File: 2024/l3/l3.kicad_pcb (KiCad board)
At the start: 2 copper layers, 137.5 x 129.1 mm, 23 parts, among them J1 Conn_01x04, SW1 SW_SPDT, SW2 SW_SPDT, SW3 SW_SPDT, SW4 SW_SPDT, U4 DEV-15583

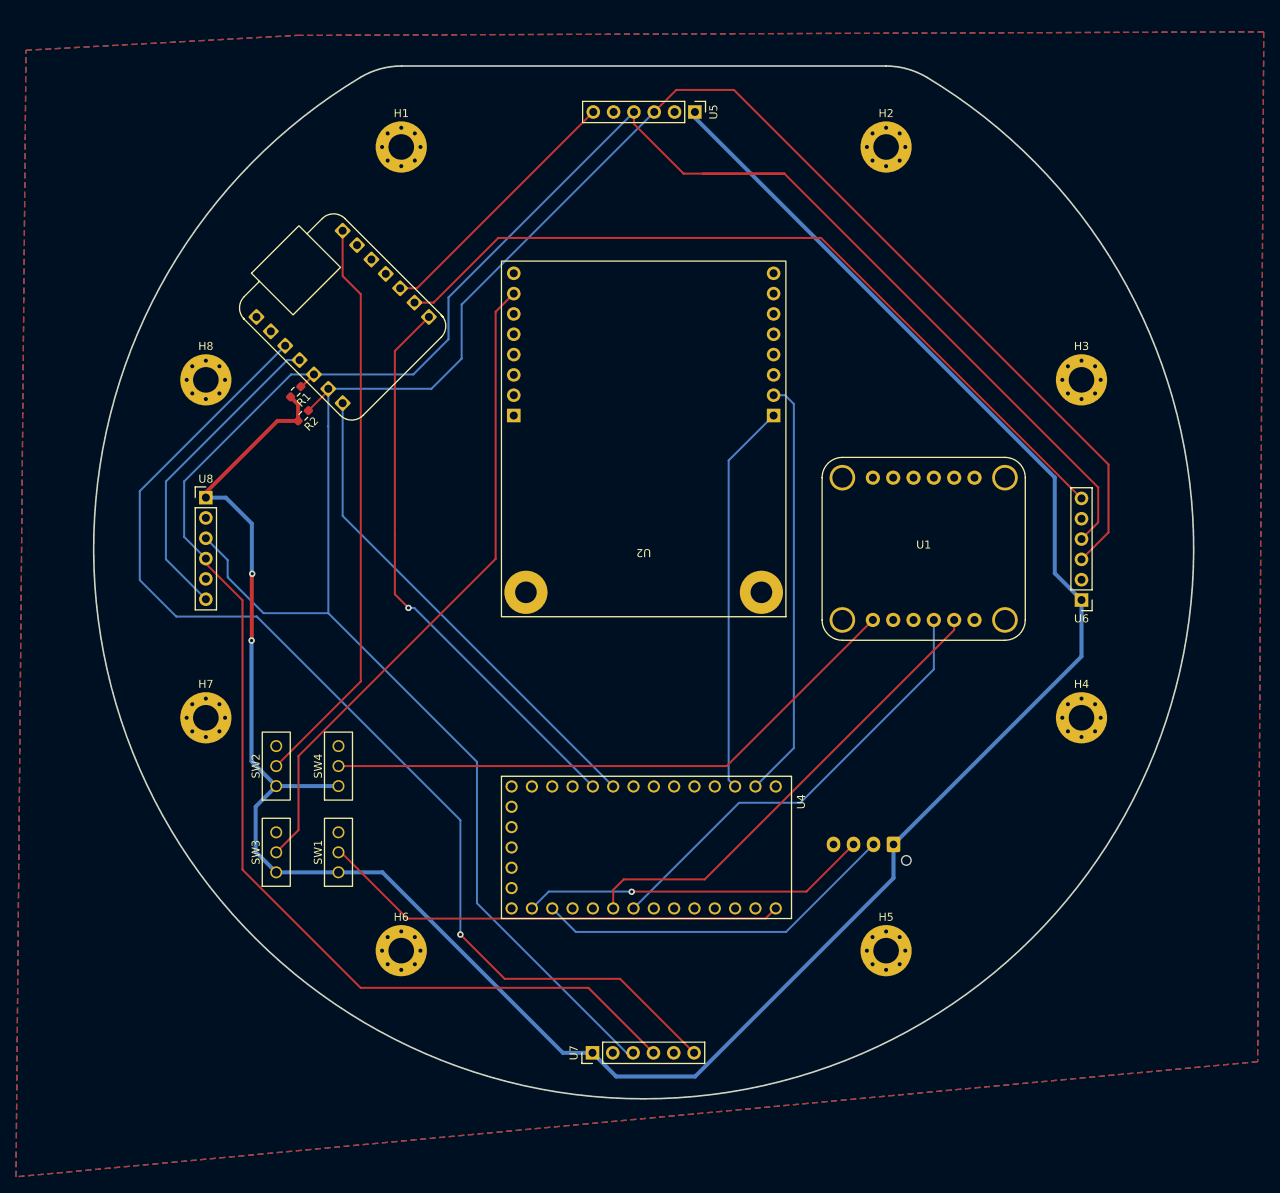
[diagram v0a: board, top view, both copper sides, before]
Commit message: nose
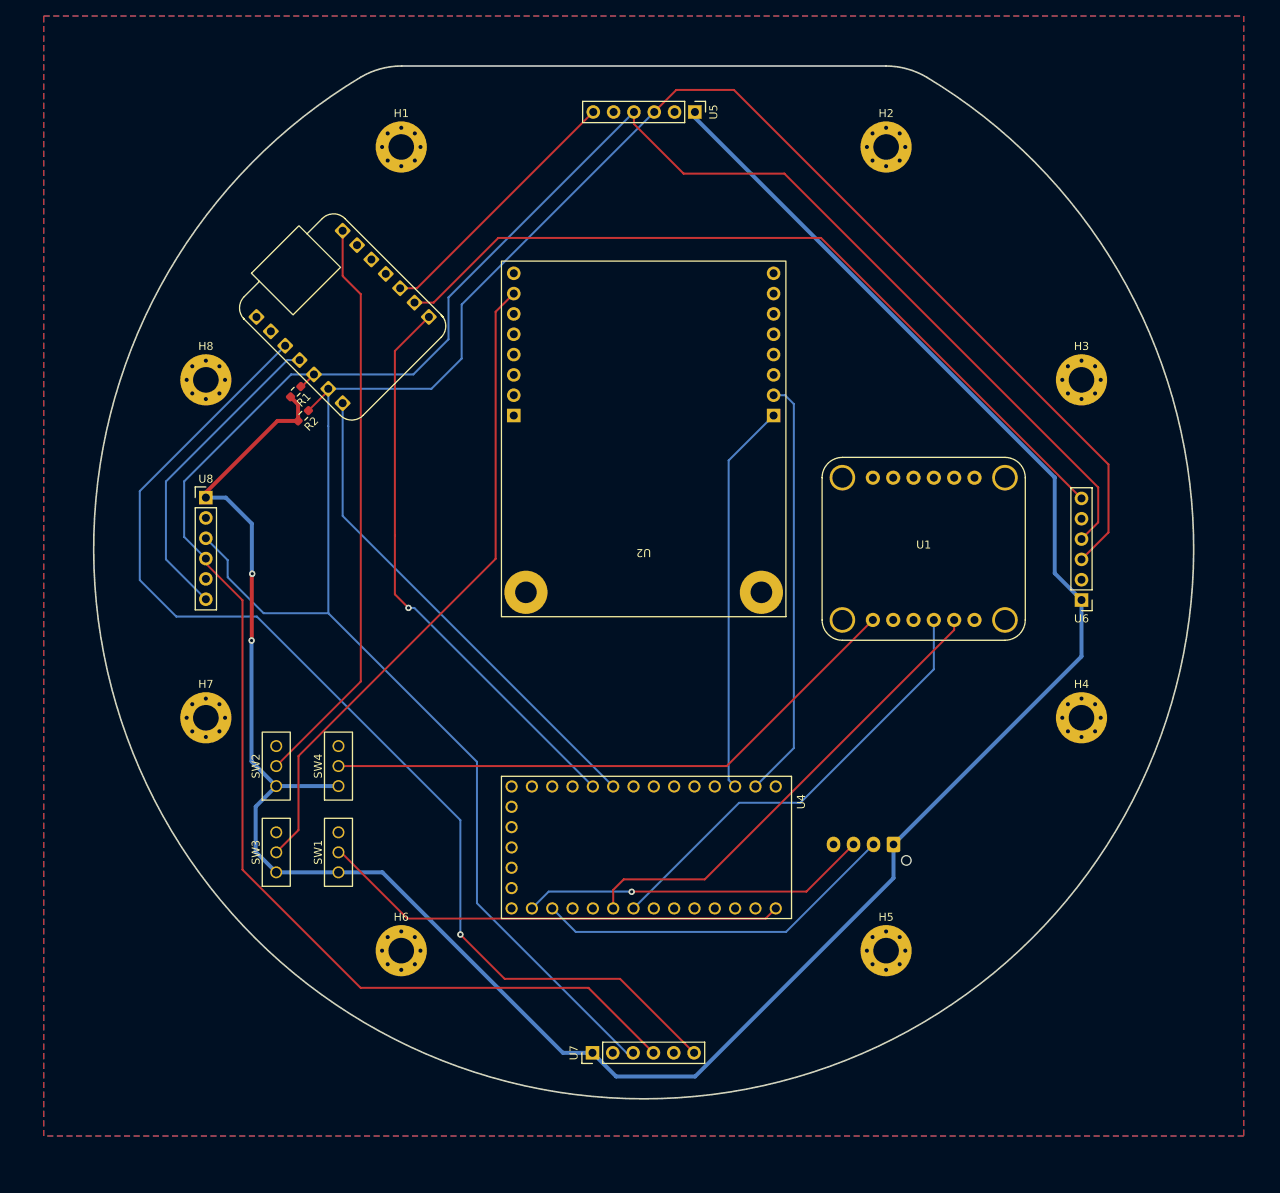
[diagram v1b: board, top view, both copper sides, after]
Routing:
- net /SDAToF: track 289.0 -> 278.8 mm
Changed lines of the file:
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@@
-	)
-	(segment
-		(start 122.59 49.7)
-		(end 112.358751 49.7)
-		(width 0.25)
-		(layer "F.Cu")
-		(net 5)
 	)
 	(segment
@@
 		(polygon
 			(pts
-				(xy 61.73 32.42) (xy 182.51 31.98) (xy 181.75 160.71) (xy 26.54 175.1) (xy 27.79 34.28)
+				(xy 30 30) (xy 180 30) (xy 180 170) (xy 30 170)
 			)
 		)
